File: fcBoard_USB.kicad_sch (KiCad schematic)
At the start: 14 parts, among them J2 USB_A, J3 USB_A, J4 USB_A, J5 USB_A, U10 TPD4S012, U11 TPS2041B, U12 TPD4S012, U13 TPS2041B, U4 TPD4S012, U5 TPS2041B, U6 USB3320, U7 USB5744, U8 TPD4S012, U9 TPS2041B

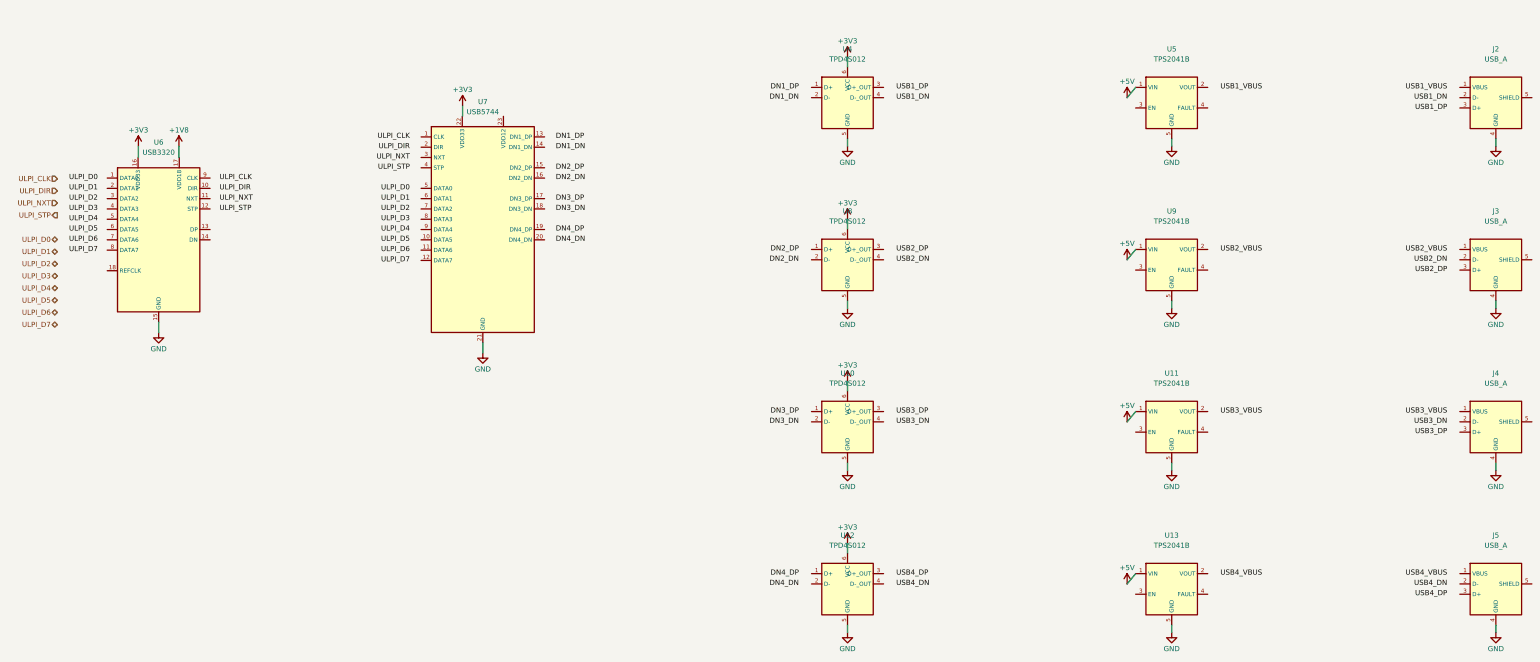
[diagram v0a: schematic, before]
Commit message: 45
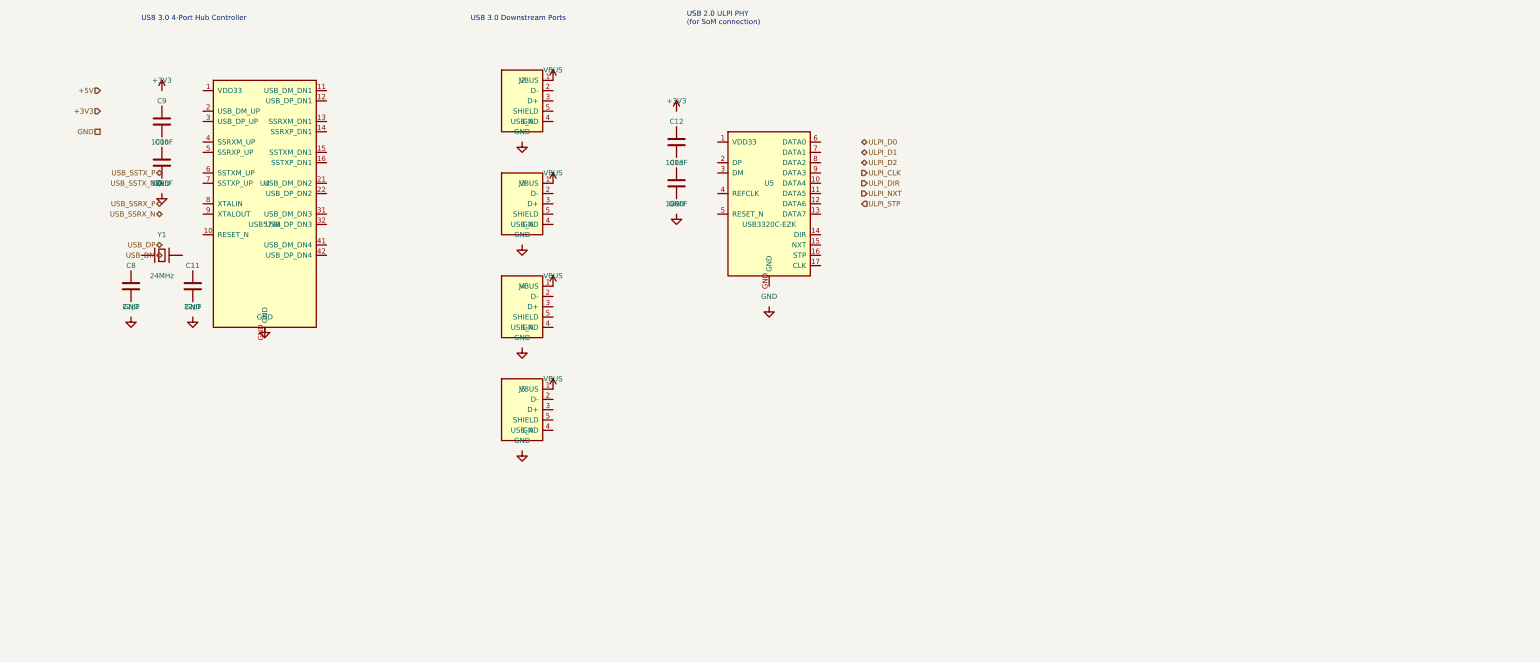
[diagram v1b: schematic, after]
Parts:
- removed J2, J3, J4, J5: USB_A, Connector_USB:USB_A_Stewart_SS-52100-001_Horizontal, symbol USB_A
- removed U10, U12, U4, U8: TPD4S012, Package_DFN_QFN:UQFN-10_1.4x1.8mm_P0.4mm, symbol TPD4S012
- removed U11, U13, U5, U9: TPS2041B, Package_TO_SOT_SMD:SOT-23-5, symbol TPS2041B
- removed U6: USB3320, Package_DFN_QFN:QFN-32-1EP_5x5mm_P0.5mm_EP3.1x3.1mm, symbol USB3320
- removed U7: USB5744, Package_DFN_QFN:QFN-48-1EP_6x6mm_P0.4mm_EP4.25x4.25mm, symbol USB5744
- added C10, C12, C13, C9: 100nF, jlc_components:C0402, symbol fcBoard:C
- added C11, C8: 22pF, jlc_components:C0402, symbol fcBoard:C
- added J2, J3, J4, J5: USB_A, jlc_components:USB-A-TH_USB-A-F-90, symbol fcBoard:USB_A
- added U4: USB5744, Package_DFN_QFN:QFN-56-1EP_7x7mm_P0.4mm_EP5.6x5.6mm, symbol fcBoard:USB5744
- added U5: USB3320C-EZK, Package_DFN_QFN:QFN-32-1EP_5x5mm_P0.5mm_EP3.6x3.6mm, symbol fcBoard:USB3320
- added Y1: 24MHz, jlc_components:HC-49S_L11.0-W4.6, symbol fcBoard:Crystal
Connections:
- new net VBUS: J2.1 (VBUS), J3.1 (VBUS), J4.1 (VBUS), J5.1 (VBUS)
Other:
- note added: "USB 2.0 ULPI PHY (for SoM connection)"
- note added: "USB 3.0 4-Port Hub Controller"
- note added: "USB 3.0 Downstream Ports"
- company: fcBoard -> fcBoard Project
- title: USB Subsystem -> USB 3.0 Hub Subsystem

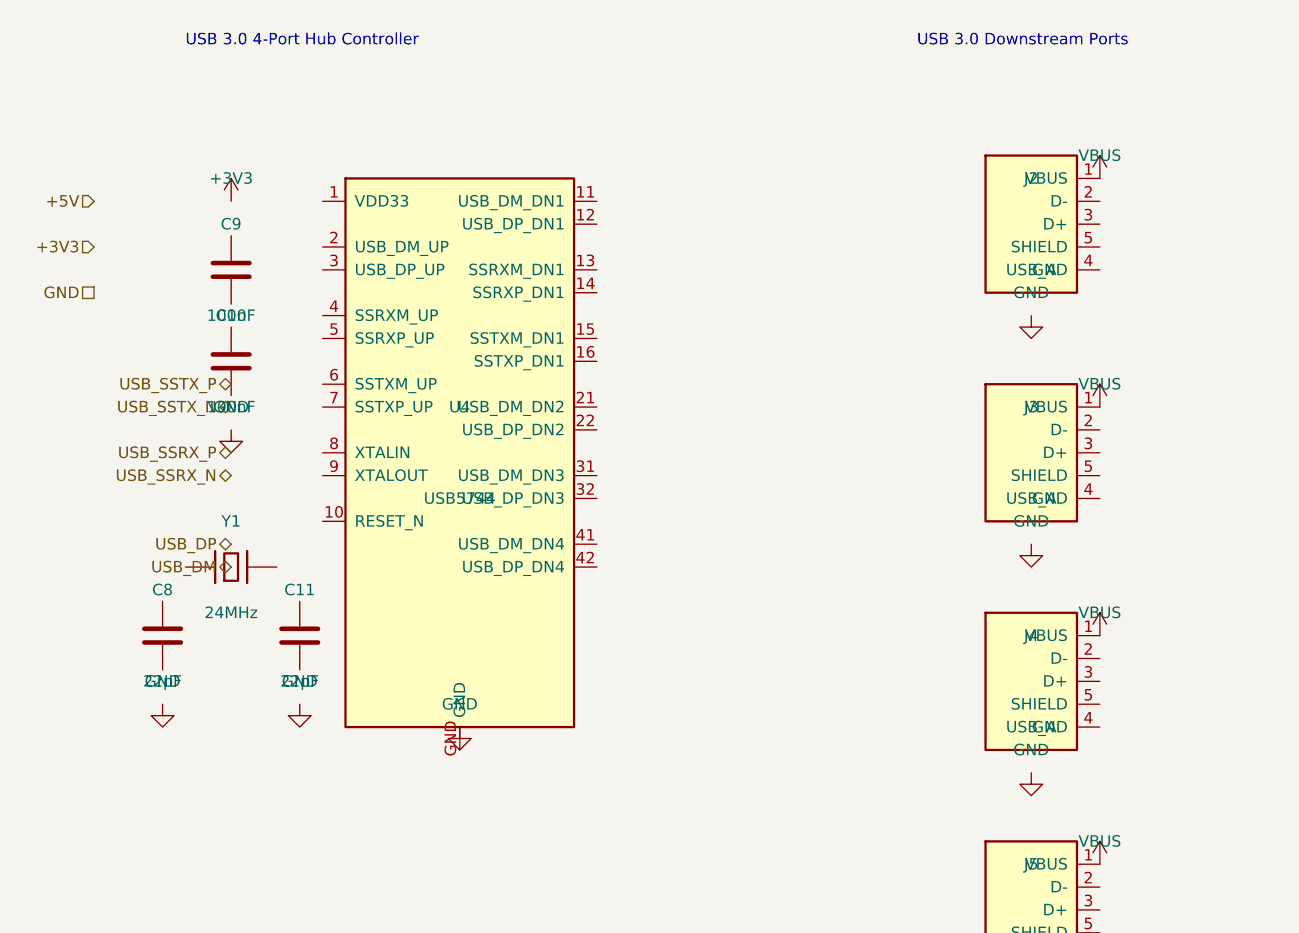
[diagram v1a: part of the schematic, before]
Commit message: 자동화
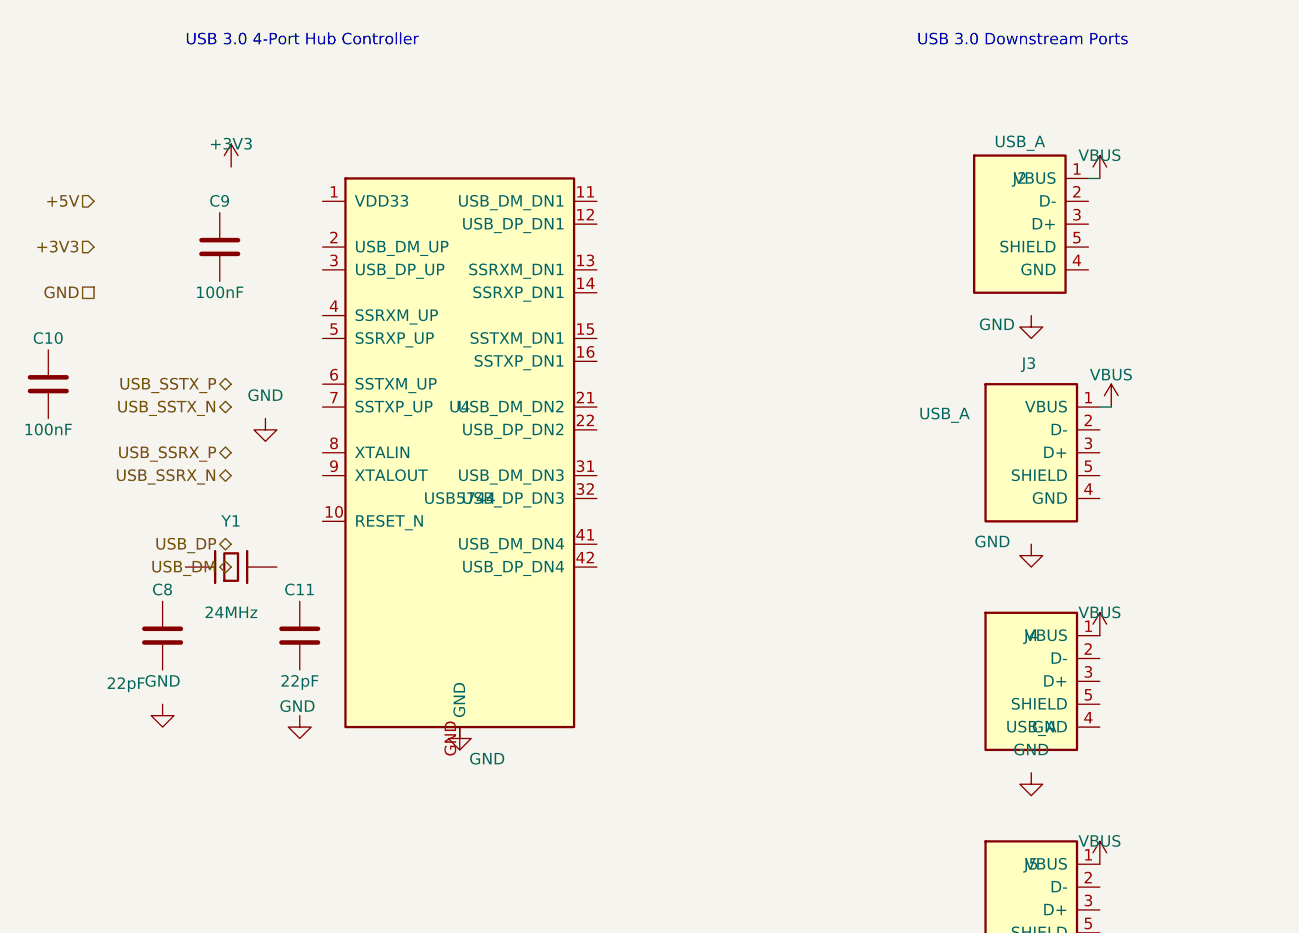
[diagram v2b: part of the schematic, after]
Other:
- moved on the sheet: C10, C9, J2
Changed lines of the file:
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@@
+		)
+	)
+	(wire
+		(pts
+			(xy 148.59 71.12) (xy 147.32 71.12)
+		)
+		(stroke
+			(width 0)
+			(type default)
+		)
+	)
+	(wire
+		(pts
+			(xy 146.05 45.72) (xy 147.32 45.72)
+		)
+		(stroke
+			(width 0)
+			(type default)
 		)
 	)
@@
 		)
 		(property "Value" "GND"
-			(at 76.2 104.14 0)
+			(at 79.248 110.236 0)
 			(effects
 				(font
@@
 	(symbol
 		(lib_id "fcBoard:USB_A")
-		(at 139.7 50.8 0)
+		(at 138.43 50.8 0)
 		(unit 1)
 		(exclude_from_sim no)
@@
 		(dnp no)
 		(property "Reference" "J2"
-			(at 139.7 45.72 0)
+			(at 138.43 45.72 0)
 			(effects
 				(font
@@
 		)
 		(property "Value" "USB_A"
-			(at 139.7 55.88 0)
+			(at 138.43 41.656 0)
 			(effects
 				(font
@@
 		)
 		(property "Footprint" "jlc_components:USB-A-TH_USB-A-F-90"
-			(at 139.7 50.8 0)
-			(effects
-				(font
-					(size 1.27 1.27)
-				)
-				(hide yes)
-			)
-		)
-		(property "Datasheet" ""
-			(at 139.7 50.8 0)
+			(at 138.43 50.8 0)
+			(effects
+				(font
+					(size 1.27 1.27)
+				)
+				(hide yes)
+			)
+		)
+		(property "Datasheet" ""
+			(at 138.43 50.8 0)
 			(effects
 				(font
@@
 		)
 		(property "Description" "USB Type-A Receptacle"
-			(at 139.7 50.8 0)
+			(at 138.43 50.8 0)
 			(effects
 				(font
@@
 		)
 		(property "LCSC Part" "C46406"
-			(at 139.7 50.8 0)
+			(at 138.43 50.8 0)
 			(effects
 				(font
@@
 	(symbol
 		(lib_id "fcBoard:GND")
-		(at 58.42 104.14 0)
+		(at 58.42 105.41 0)
 		(unit 1)
 		(exclude_from_sim no)
@@
 		(dnp no)
 		(property "Reference" "#PWR033"
-			(at 58.42 106.68 0)
+			(at 58.42 107.95 0)
 			(effects
 				(font
@@
 		)
 		(property "Value" "GND"
-			(at 58.42 101.6 0)
+			(at 58.166 104.394 0)
 			(effects
 				(font
@@
 		)
 		(property "Footprint" ""
-			(at 58.42 104.14 0)
-			(effects
-				(font
-					(size 1.27 1.27)
-				)
-				(hide yes)
-			)
-		)
-		(property "Datasheet" ""
-			(at 58.42 104.14 0)
+			(at 58.42 105.41 0)
+			(effects
+				(font
+					(size 1.27 1.27)
+				)
+				(hide yes)
+			)
+		)
+		(property "Datasheet" ""
+			(at 58.42 105.41 0)
 			(effects
 				(font
@@
 		)
 		(property "Description" "Power Ground"
-			(at 58.42 104.14 0)
+			(at 58.42 105.41 0)
 			(effects
 				(font
@@
 		)
 		(property "Value" "GND"
-			(at 139.7 83.82 0)
+			(at 135.382 86.106 0)
 			(effects
 				(font
@@
 		(dnp no)
 		(property "Reference" "J3"
-			(at 139.7 71.12 0)
+			(at 139.446 66.294 0)
 			(effects
 				(font
@@
 		)
 		(property "Value" "USB_A"
-			(at 139.7 81.28 0)
+			(at 130.048 71.882 0)
 			(effects
 				(font
@@
 		)
 		(property "Value" "22pF"
-			(at 43.18 101.6 0)
+			(at 39.116 101.854 0)
 			(effects
 				(font
@@
 	(symbol
 		(lib_id "fcBoard:GND")
-		(at 50.8 73.66 0)
+		(at 54.61 72.39 0)
 		(unit 1)
 		(exclude_from_sim no)
@@
 		(dnp no)
 		(property "Reference" "#PWR032"
-			(at 50.8 76.2 0)
+			(at 54.61 74.93 0)
 			(effects
 				(font
@@
 		)
 		(property "Value" "GND"
-			(at 50.8 71.12 0)
+			(at 54.61 69.85 0)
 			(effects
 				(font
@@
 		)
 		(property "Footprint" ""
-			(at 50.8 73.66 0)
-			(effects
-				(font
-					(size 1.27 1.27)
-				)
-				(hide yes)
-			)
-		)
-		(property "Datasheet" ""
-			(at 50.8 73.66 0)
+			(at 54.61 72.39 0)
+			(effects
+				(font
+					(size 1.27 1.27)
+				)
+				(hide yes)
+			)
+		)
+		(property "Datasheet" ""
+			(at 54.61 72.39 0)
 			(effects
 				(font
@@
 		)
 		(property "Description" "Power Ground"
-			(at 50.8 73.66 0)
+			(at 54.61 72.39 0)
 			(effects
 				(font
@@
 	(symbol
 		(lib_id "fcBoard:VBUS")
-		(at 147.32 71.12 0)
+		(at 148.59 71.12 0)
 		(unit 1)
 		(exclude_from_sim no)
@@
 		(dnp no)
 		(property "Reference" "#PWR040"
-			(at 147.32 73.66 0)
+			(at 148.59 73.66 0)
 			(effects
 				(font
@@
 		)
 		(property "Value" "VBUS"
-			(at 147.32 68.58 0)
+			(at 148.59 67.564 0)
 			(effects
 				(font
@@
 		)
 		(property "Footprint" ""
-			(at 147.32 71.12 0)
-			(effects
-				(font
-					(size 1.27 1.27)
-				)
-				(hide yes)
-			)
-		)
-		(property "Datasheet" ""
-			(at 147.32 71.12 0)
+			(at 148.59 71.12 0)
+			(effects
+				(font
+					(size 1.27 1.27)
+				)
+				(hide yes)
+			)
+		)
+		(property "Datasheet" ""
+			(at 148.59 71.12 0)
 			(effects
 				(font
@@
 		)
 		(property "Description" "USB VBUS Power"
-			(at 147.32 71.12 0)
+			(at 148.59 71.12 0)
 			(effects
 				(font
@@
 	(symbol
 		(lib_id "fcBoard:C")
-		(at 50.8 55.88 0)
+		(at 49.53 53.34 0)
 		(unit 1)
 		(exclude_from_sim no)
@@
 		(dnp no)
 		(property "Reference" "C9"
-			(at 50.8 50.8 0)
+			(at 49.53 48.26 0)
 			(effects
 				(font
@@
 		)
 		(property "Value" "100nF"
-			(at 50.8 60.96 0)
+			(at 49.53 58.42 0)
 			(effects
 				(font
@@
 		)
 		(property "Footprint" "jlc_components:C0402"
-			(at 50.8 55.88 0)
-			(effects
-				(font
-					(size 1.27 1.27)
-				)
-				(hide yes)
-			)
-		)
-		(property "Datasheet" ""
-			(at 50.8 55.88 0)
+			(at 49.53 53.34 0)
+			(effects
+				(font
+					(size 1.27 1.27)
+				)
+				(hide yes)
+			)
+		)
+		(property "Datasheet" ""
+			(at 49.53 53.34 0)
 			(effects
 				(font
@@
 		)
 		(property "Description" "Capacitor"
-			(at 50.8 55.88 0)
+			(at 49.53 53.34 0)
 			(effects
 				(font
@@
 		)
 		(property "LCSC Part" "C11702"
-			(at 50.8 55.88 0)
+			(at 49.53 53.34 0)
 			(effects
 				(font
@@
 	(symbol
 		(lib_id "fcBoard:C")
-		(at 50.8 66.04 0)
+		(at 30.48 68.58 0)
 		(unit 1)
 		(exclude_from_sim no)
@@
 		(dnp no)
 		(property "Reference" "C10"
-			(at 50.8 60.96 0)
+			(at 30.48 63.5 0)
 			(effects
 				(font
@@
 		)
 		(property "Value" "100nF"
-			(at 50.8 71.12 0)
+			(at 30.48 73.66 0)
 			(effects
 				(font
@@
 		)
 		(property "Footprint" "jlc_components:C0402"
-			(at 50.8 66.04 0)
-			(effects
-				(font
-					(size 1.27 1.27)
-				)
-				(hide yes)
-			)
-		)
-		(property "Datasheet" ""
-			(at 50.8 66.04 0)
+			(at 30.48 68.58 0)
+			(effects
+				(font
+					(size 1.27 1.27)
+				)
+				(hide yes)
+			)
+		)
+		(property "Datasheet" ""
+			(at 30.48 68.58 0)
 			(effects
 				(font
@@
 		)
 		(property "Description" "Capacitor"
-			(at 50.8 66.04 0)
+			(at 30.48 68.58 0)
 			(effects
 				(font
@@
 		)
 		(property "LCSC Part" "C11702"
-			(at 50.8 66.04 0)
+			(at 30.48 68.58 0)
 			(effects
 				(font
@@
 		)
 		(property "Value" "GND"
-			(at 139.7 58.42 0)
+			(at 135.89 61.976 0)
 			(effects
 				(font
@@
 	(symbol
 		(lib_id "fcBoard:+3V3")
-		(at 50.8 48.26 0)
+		(at 50.8 44.45 0)
 		(unit 1)
 		(exclude_from_sim no)
@@
 		(dnp no)
 		(property "Reference" "#PWR031"
-			(at 50.8 50.8 0)
+			(at 50.8 46.99 0)
 			(effects
 				(font
@@
 		)
 		(property "Value" "+3V3"
-			(at 50.8 45.72 0)
+			(at 50.8 41.91 0)
 			(effects
 				(font
@@
 		)
 		(property "Footprint" ""
-			(at 50.8 48.26 0)
-			(effects
-				(font
-					(size 1.27 1.27)
-				)
-				(hide yes)
-			)
-		)
-		(property "Datasheet" ""
-			(at 50.8 48.26 0)
+			(at 50.8 44.45 0)
+			(effects
+				(font
+					(size 1.27 1.27)
+				)
+				(hide yes)
+			)
+		)
+		(property "Datasheet" ""
+			(at 50.8 44.45 0)
 			(effects
 				(font
@@
 		)
 		(property "Description" "+3.3V Power Rail"
-			(at 50.8 48.26 0)
-			(effects
-				(font
+			(at 50.8 44.45 0)
+			(effects
+				(font
